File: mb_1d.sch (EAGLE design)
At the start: 57 parts, among them CON1 1013279X_AMPHENOL_2X25, CON2 1013279X_AMPHENOL_2X25, U1 TPS61040, U10 TPS610981, U2 MAX5394, U3 TPS61040, U4 74HC4050, U5 RFD77101, U6 MAX5394, U7 MAX5026EUT+T, U8 MAX5394

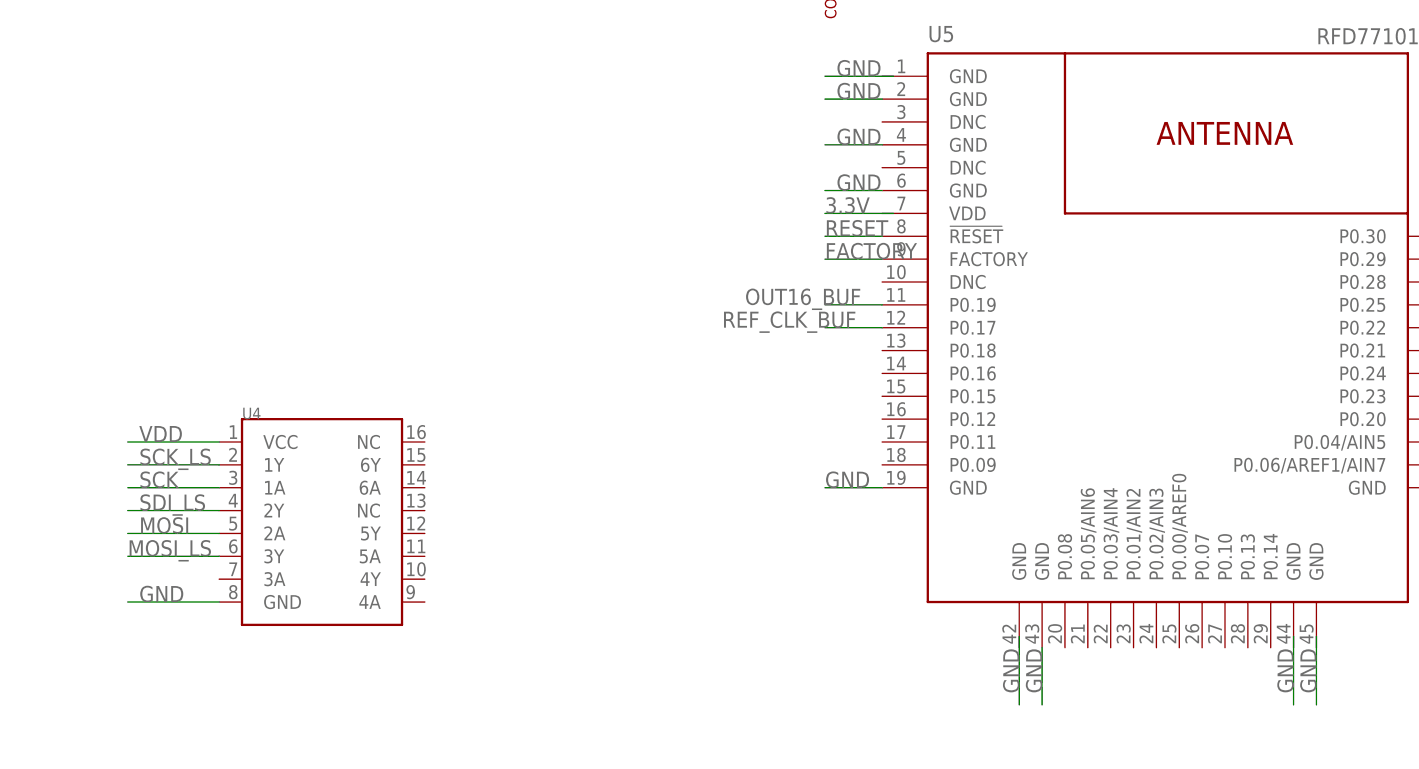
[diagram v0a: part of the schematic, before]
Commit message: Began schematic
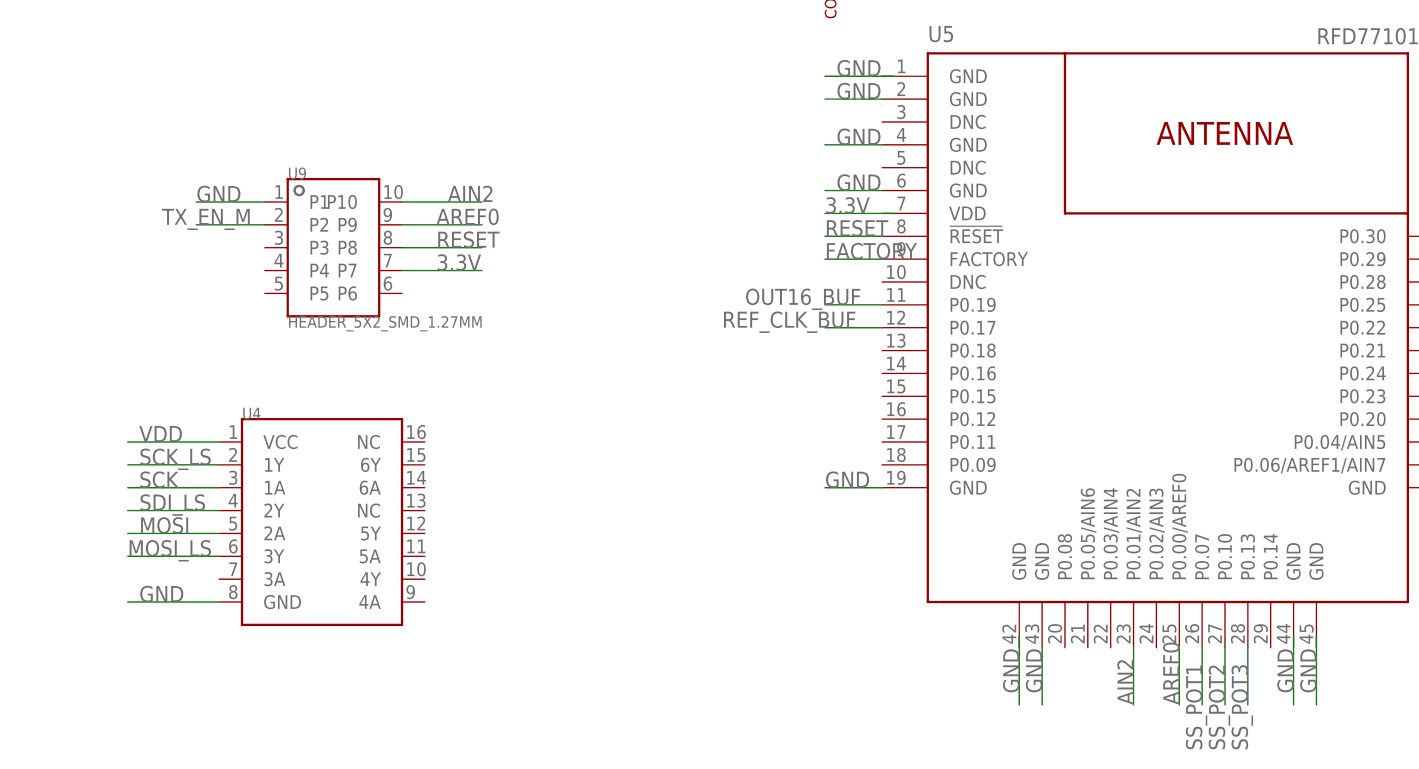
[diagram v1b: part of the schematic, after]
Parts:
- added U9: HEADER_5X2_SMD_1.27MM, ck:HEADER_5X2_SMD_1.27MM
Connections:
- new net AIN2: U5.P0.01/AIN2, U9.P10
- new net AREF0: U5.P0.00/AREF0, U9.P9
- net 3.3V: now also U9.P7
- net GND: now also U9.P1
- net RESET: now also U9.P8
- net SS_POT1: now also U5.P0.07
- net SS_POT2: now also U5.P0.10
- net SS_POT3: now also U5.P0.13
- net TX_EN_M: now also U9.P2
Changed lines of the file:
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@@
 <part name="U8" library="ck" deviceset="MAX5394" device=""/>
 <part name="R13" library="SparkFun-Resistors" deviceset="RESISTOR" device="0402" value="50k"/>
+<part name="U9" library="ck" deviceset="HEADER_5X2_SMD_1.27MM" device=""/>
 </parts>
 <sheets>
@@
 <instance part="U8" gate="U1" x="-95.25" y="-35.56"/>
 <instance part="R13" gate="G$1" x="-80.01" y="-49.53" rot="R90"/>
+<instance part="U9" gate="U1" x="29.21" y="-64.77"/>
 </instances>
 <busses>
@@
 <label x="-80.01" y="-59.69" size="1.778" layer="95"/>
 </segment>
+<segment>
+<pinref part="U9" gate="U1" pin="P1"/>
+<wire x1="21.59" y1="-58.42" x2="13.97" y2="-58.42" width="0.1524" layer="91"/>
+<label x="13.97" y="-58.42" size="1.778" layer="95"/>
+</segment>
 </net>
 <net name="3.3V" class="0">
@@
 <label x="-113.03" y="-27.94" size="1.778" layer="95"/>
 </segment>
+<segment>
+<pinref part="U9" gate="U1" pin="P7"/>
+<wire x1="36.83" y1="-66.04" x2="45.72" y2="-66.04" width="0.1524" layer="91"/>
+<label x="40.64" y="-66.04" size="1.778" layer="95"/>
+</segment>
 </net>
 <net name="SCK" class="0">
@@
 <pinref part="CON2" gate="CON1" pin="P$41"/>
 </segment>
+<segment>
+<pinref part="U9" gate="U1" pin="P2"/>
+<wire x1="21.59" y1="-60.96" x2="13.97" y2="-60.96" width="0.1524" layer="91"/>
+<label x="10.16" y="-60.96" size="1.778" layer="95"/>
+</segment>
 </net>
 <net name="RSTB_M" class="0">
@@
 <wire x1="90.17" y1="-62.23" x2="83.82" y2="-62.23" width="0.1524" layer="91"/>
 <label x="83.82" y="-62.23" size="1.778" layer="95"/>
+</segment>
+<segment>
+<pinref part="U9" gate="U1" pin="P8"/>
+<wire x1="36.83" y1="-63.5" x2="45.72" y2="-63.5" width="0.1524" layer="91"/>
+<label x="40.64" y="-63.5" size="1.778" layer="95"/>
 </segment>
 </net>
@@
 <label x="12.7" y="25.4" size="1.778" layer="95"/>
 </segment>
+<segment>
+<pinref part="U5" gate="G$1" pin="P0.07"/>
+<wire x1="125.73" y1="-107.95" x2="125.73" y2="-114.3" width="0.1524" layer="91"/>
+<label x="125.73" y="-119.38" size="1.778" layer="95" rot="R90"/>
+</segment>
 </net>
 <net name="SS_POT2" class="0">
@@
 <wire x1="-224.79" y1="-36.83" x2="-233.68" y2="-36.83" width="0.1524" layer="91"/>
 <label x="-237.49" y="-36.83" size="1.778" layer="95"/>
+</segment>
+<segment>
+<pinref part="U5" gate="G$1" pin="P0.10"/>
+<wire x1="128.27" y1="-107.95" x2="128.27" y2="-114.3" width="0.1524" layer="91"/>
+<label x="128.27" y="-119.38" size="1.778" layer="95" rot="R90"/>
 </segment>
 </net>
@@
 <label x="-118.11" y="-33.02" size="1.778" layer="95"/>
 </segment>
+<segment>
+<pinref part="U5" gate="G$1" pin="P0.13"/>
+<wire x1="130.81" y1="-107.95" x2="130.81" y2="-114.3" width="0.1524" layer="91"/>
+<label x="130.81" y="-119.38" size="1.778" layer="95" rot="R90"/>
+</segment>
 </net>
 <net name="MOSI_LS" class="0">
@@
 </segment>
 </net>
+<net name="AIN2" class="0">
+<segment>
+<pinref part="U9" gate="U1" pin="P10"/>
+<wire x1="36.83" y1="-58.42" x2="45.72" y2="-58.42" width="0.1524" layer="91"/>
+<label x="41.91" y="-58.42" size="1.778" layer="95"/>
+</segment>
+<segment>
+<pinref part="U5" gate="G$1" pin="P0.01/AIN2"/>
+<wire x1="118.11" y1="-107.95" x2="118.11" y2="-114.3" width="0.1524" layer="91"/>
+<label x="118.11" y="-114.3" size="1.778" layer="95" rot="R90"/>
+</segment>
+</net>
+<net name="AREF0" class="0">
+<segment>
+<pinref part="U9" gate="U1" pin="P9"/>
+<wire x1="36.83" y1="-60.96" x2="45.72" y2="-60.96" width="0.1524" layer="91"/>
+<label x="40.64" y="-60.96" size="1.778" layer="95"/>
+</segment>
+<segment>
+<pinref part="U5" gate="G$1" pin="P0.00/AREF0"/>
+<wire x1="123.19" y1="-107.95" x2="123.19" y2="-114.3" width="0.1524" layer="91"/>
+<label x="123.19" y="-114.3" size="1.778" layer="95" rot="R90"/>
+</segment>
+</net>
